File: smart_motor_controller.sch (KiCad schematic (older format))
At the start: 76 parts, among them J1 I2C_CONN_1, J10 USB_B_Micro, J11 M0_CONN, J12 M1_CONN, J13 M2_CONN, J14 M3_CONN, J2 I2C_CONN_2, J3 Conn_01x02, J4 Conn_02x05_Odd_Even, J5 Conn_01x02, J6 Conn_01x02, J7 Conn_01x02, J8 CAN_CONN, J9 Input 12V, Q1 AO3401A, SW1 SW_SPDT, U1 TPS5430DDA, U2 STM32F405RGT6, U3 USBLC6-2SC6, U4 DRV8871DDA, U5 DRV8871DDA, U6 DRV8871DDA, U7 DRV8871DDA

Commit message: V0.1.1 Removed fuse and AO3401A
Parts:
- removed F1: Polyfuse, Fuse:Fuse_1812_4532Metric, symbol Device:Polyfuse_Small
- removed Q1: AO3401A, Package_TO_SOT_SMD:SOT-23, symbol Transistor_FET:AO3401A
- R2, R3: footprint Resistor_SMD:R_0402_1005Metric -> Resistor_THT:R_Axial_DIN0204_L3.6mm_D1.6mm_P5.08mm_Horizontal; LCSC Part # C25879 -> (none)
- TP1: value 12V -> Vin
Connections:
- wire segments 172 -> 170
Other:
- moved on the sheet: C1, D1, D2, TP1
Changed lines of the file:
@@
 NoConn ~ 10800 1150
-$Comp
-L power:+12V #PWR0101
-U 1 1 602FED4E
-P 700 1000
-F 0 "#PWR0101" H 700 850 50  0001 C CNN
-F 1 "+12V" H 715 1173 50  0000 C CNN
-F 2 "" H 700 1000 50  0001 C CNN
-F 3 "" H 700 1000 50  0001 C CNN
-	1    700  1000
-	1    0    0    -1
-$EndComp
-$Comp
-L Device:Polyfuse_Small F1
-U 1 1 602FF711
-P 1500 1150
-F 0 "F1" V 1295 1150 50  0000 C CNN
-F 1 "Polyfuse" V 1386 1150 50  0000 C CNN
-F 2 "Fuse:Fuse_1812_4532Metric" H 1550 950 50  0001 L CNN
-F 3 "~" H 1500 1150 50  0001 C CNN
-F 4 "C495356" H 1500 1150 50  0001 C CNN "LCSC Part #"
-	1    1500 1150
-	0    1    1    0
-$EndComp
 $Comp
 L Connector:Screw_Terminal_01x02 J9
@@
 L power:+5V #PWR0110
 U 1 1 6038E68B
-P 2050 800
-F 0 "#PWR0110" H 2050 650 50  0001 C CNN
-F 1 "+5V" H 2065 973 50  0000 C CNN
-F 2 "" H 2050 800 50  0001 C CNN
-F 3 "" H 2050 800 50  0001 C CNN
-	1    2050 800
+P 1800 1050
+F 0 "#PWR0110" H 1800 900 50  0001 C CNN
+F 1 "+5V" H 1815 1223 50  0000 C CNN
+F 2 "" H 1800 1050 50  0001 C CNN
+F 3 "" H 1800 1050 50  0001 C CNN
+	1    1800 1050
 	1    0    0    -1
 $EndComp
@@
 F 0 "R2" H 4309 5646 50  0000 L CNN
 F 1 "2k2" H 4309 5555 50  0000 L CNN
-F 2 "Resistor_SMD:R_0402_1005Metric" H 4250 5600 50  0001 C CNN
+F 2 "Resistor_THT:R_Axial_DIN0204_L3.6mm_D1.6mm_P5.08mm_Horizontal" H 4250 5600 50  0001 C CNN
 F 3 "~" H 4250 5600 50  0001 C CNN
-F 4 "C25879" H 4250 5600 50  0001 C CNN "LCSC Part #"
+F 4 "" H 4250 5600 50  0001 C CNN "LCSC Part #"
 	1    4250 5600
 	1    0    0    -1
@@
 F 0 "R3" H 4609 5646 50  0000 L CNN
 F 1 "2k2" H 4609 5555 50  0000 L CNN
-F 2 "Resistor_SMD:R_0402_1005Metric" H 4550 5600 50  0001 C CNN
+F 2 "Resistor_THT:R_Axial_DIN0204_L3.6mm_D1.6mm_P5.08mm_Horizontal" H 4550 5600 50  0001 C CNN
 F 3 "~" H 4550 5600 50  0001 C CNN
-F 4 "C25879" H 4550 5600 50  0001 C CNN "LCSC Part #"
+F 4 "" H 4550 5600 50  0001 C CNN "LCSC Part #"
 	1    4550 5600
 	1    0    0    -1
@@
 L Device:C_Small C1
 U 1 1 60354332
-P 2250 1350
-F 0 "C1" H 2342 1396 50  0000 L CNN
-F 1 "10u" H 2342 1305 50  0000 L CNN
-F 2 "Capacitor_SMD:C_1206_3216Metric" H 2250 1350 50  0001 C CNN
-F 3 "~" H 2250 1350 50  0001 C CNN
-F 4 "C13585" H 2250 1350 50  0001 C CNN "LCSC Part #"
-	1    2250 1350
+P 2000 1600
+F 0 "C1" H 2092 1646 50  0000 L CNN
+F 1 "10u" H 2092 1555 50  0000 L CNN
+F 2 "Capacitor_SMD:C_1206_3216Metric" H 2000 1600 50  0001 C CNN
+F 3 "~" H 2000 1600 50  0001 C CNN
+F 4 "C13585" H 2000 1600 50  0001 C CNN "LCSC Part #"
+	1    2000 1600
 	1    0    0    -1
 $EndComp
@@
 Text GLabel 4200 1000 0    50   Input ~ 0
 BACK_IN
-Text GLabel 2400 1150 2    50   Input ~ 0
+Text GLabel 2150 1400 2    50   Input ~ 0
 BACK_IN
 $Comp
 L power:GND #PWR0117
 U 1 1 6037A407
-P 2250 1450
-F 0 "#PWR0117" H 2250 1200 50  0001 C CNN
-F 1 "GND" H 2255 1277 50  0000 C CNN
-F 2 "" H 2250 1450 50  0001 C CNN
-F 3 "" H 2250 1450 50  0001 C CNN
-	1    2250 1450
-	1    0    0    -1
-$EndComp
-Wire Wire Line
-	2400 1150 2250 1150
-Wire Wire Line
-	2250 1150 2250 1250
+P 2000 1700
+F 0 "#PWR0117" H 2000 1450 50  0001 C CNN
+F 1 "GND" H 2005 1527 50  0000 C CNN
+F 2 "" H 2000 1700 50  0001 C CNN
+F 3 "" H 2000 1700 50  0001 C CNN
+	1    2000 1700
+	1    0    0    -1
+$EndComp
+Wire Wire Line
+	2150 1400 2000 1400
+Wire Wire Line
+	2000 1400 2000 1500
 Text GLabel 3300 850  0    50   Input ~ 0
 BACK_IN
@@
 Wire Wire Line
 	3800 3800 3950 3800
-Wire Wire Line
-	700  1000 700  1150
-Connection ~ 2250 1150
+Connection ~ 2000 1400
 $Comp
 L Device:D_Schottky_Small D1
 U 1 1 603C17FB
-P 2050 1000
-F 0 "D1" V 2250 850 50  0000 L CNN
-F 1 "B5819W" V 2150 650 50  0000 L CNN
-F 2 "Diode_SMD:D_SOD-123" V 2050 1000 50  0001 C CNN
-F 3 "~" V 2050 1000 50  0001 C CNN
-F 4 "C8598" H 2050 1000 50  0001 C CNN "LCSC Part #"
-	1    2050 1000
+P 1800 1250
+F 0 "D1" V 2000 1100 50  0000 L CNN
+F 1 "B5819W" V 1900 900 50  0000 L CNN
+F 2 "Diode_SMD:D_SOD-123" V 1800 1250 50  0001 C CNN
+F 3 "~" V 1800 1250 50  0001 C CNN
+F 4 "C8598" H 1800 1250 50  0001 C CNN "LCSC Part #"
+	1    1800 1250
 	0    -1   -1   0
 $EndComp
 Wire Wire Line
-	2050 1100 2050 1150
-Wire Wire Line
-	2050 1150 2250 1150
-Wire Wire Line
-	2050 800  2050 900
+	1800 1350 1800 1400
+Wire Wire Line
+	1800 1400 2000 1400
+Wire Wire Line
+	1800 1050 1800 1150
 Text GLabel 10200 4150 2    50   Input ~ 0
 VM
@@
 	6500 4500 6500 4600
 Connection ~ 6500 4600
-Wire Wire Line
-	700  1150 850  1150
-$Comp
-L Device:D_Schottky_Small D2
-U 1 1 603C3D54
-P 1900 1150
-F 0 "D2" H 1950 1050 50  0000 L CNN
-F 1 "B5819W" H 1750 1250 50  0000 L CNN
-F 2 "Diode_SMD:D_SOD-123" V 1900 1150 50  0001 C CNN
-F 3 "~" V 1900 1150 50  0001 C CNN
-F 4 "C8598" H 1900 1150 50  0001 C CNN "LCSC Part #"
-	1    1900 1150
-	-1   0    0    1
-$EndComp
-Text GLabel 1750 1450 2    50   Input ~ 0
-VM
-Wire Wire Line
-	1600 1150 1700 1150
-Connection ~ 1700 1150
-Wire Wire Line
-	1700 1150 1800 1150
-Wire Wire Line
-	2000 1150 2050 1150
-Connection ~ 2050 1150
-Wire Wire Line
-	1700 1450 1750 1450
-Wire Wire Line
-	1700 1150 1700 1450
 Text GLabel 2900 6500 2    50   Input ~ 0
 GPIO0
@@
 	10150 5450 10150 5500
 $Comp
-L power:GND #PWR0133
-U 1 1 60394456
-P 1050 1450
-F 0 "#PWR0133" H 1050 1200 50  0001 C CNN
-F 1 "GND" H 1055 1277 50  0000 C CNN
-F 2 "" H 1050 1450 50  0001 C CNN
-F 3 "" H 1050 1450 50  0001 C CNN
-	1    1050 1450
-	1    0    0    -1
-$EndComp
-$Comp
-L Transistor_FET:AO3401A Q1
-U 1 1 6039186B
-P 1050 1250
-F 0 "Q1" V 1392 1250 50  0000 C CNN
-F 1 "AO3401A" V 1301 1250 50  0000 C CNN
-F 2 "Package_TO_SOT_SMD:SOT-23" H 1250 1175 50  0001 L CIN
-F 3 "http://www.aosmd.com/pdfs/datasheet/AO3401A.pdf" H 1050 1250 50  0001 L CNN
-F 4 "C693260" H 1050 1250 50  0001 C CNN "LCSC Part #"
-	1    1050 1250
-	0    -1   -1   0
-$EndComp
-Connection ~ 1350 1150
-Wire Wire Line
-	1350 1150 1400 1150
-Wire Wire Line
-	1250 1150 1350 1150
-Wire Wire Line
-	1350 1150 1350 1300
-$Comp
-L Connector:TestPoint_Small TP1
-U 1 1 604A4E02
-P 1350 1300
-F 0 "TP1" H 1398 1346 50  0000 L CNN
-F 1 "12V" H 1398 1255 50  0000 L CNN
-F 2 "TestPoint:TestPoint_Pad_D2.0mm" H 1550 1300 50  0001 C CNN
-F 3 "~" H 1550 1300 50  0001 C CNN
-	1    1350 1300
-	1    0    0    -1
-$EndComp
-$Comp
 L Connector:TestPoint_Small TP2
 U 1 1 606A33A8
@@
 Text GLabel 5200 1200 2    50   Input ~ 0
 BACK_PH
+$Comp
+L power:+12V #PWR0101
+U 1 1 602FED4E
+P 800 1050
+F 0 "#PWR0101" H 800 900 50  0001 C CNN
+F 1 "+12V" H 815 1223 50  0000 C CNN
+F 2 "" H 800 1050 50  0001 C CNN
+F 3 "" H 800 1050 50  0001 C CNN
+	1    800  1050
+	1    0    0    -1
+$EndComp
+Text GLabel 1100 1700 2    50   Input ~ 0
+VM
+Wire Wire Line
+	1050 1700 1100 1700
+$Comp
+L Device:D_Schottky_Small D2
+U 1 1 603C3D54
+P 1250 1400
+F 0 "D2" H 1300 1300 50  0000 L CNN
+F 1 "B5819W" H 1100 1500 50  0000 L CNN
+F 2 "Diode_SMD:D_SOD-123" V 1250 1400 50  0001 C CNN
+F 3 "~" V 1250 1400 50  0001 C CNN
+F 4 "C8598" H 1250 1400 50  0001 C CNN "LCSC Part #"
+	1    1250 1400
+	-1   0    0    1
+$EndComp
+Wire Wire Line
+	1050 1400 1150 1400
+Connection ~ 1050 1400
+Wire Wire Line
+	1050 1400 1050 1700
+$Comp
+L Connector:TestPoint_Small TP1
+U 1 1 604A4E02
+P 1600 1600
+F 0 "TP1" H 1648 1646 50  0000 L CNN
+F 1 "Vin" H 1648 1555 50  0000 L CNN
+F 2 "TestPoint:TestPoint_Pad_D2.0mm" H 1800 1600 50  0001 C CNN
+F 3 "~" H 1800 1600 50  0001 C CNN
+	1    1600 1600
+	1    0    0    -1
+$EndComp
+Wire Wire Line
+	800  1050 800  1400
+Wire Wire Line
+	1350 1400 1600 1400
+Connection ~ 1800 1400
+Wire Wire Line
+	1600 1600 1600 1400
+Connection ~ 1600 1400
+Wire Wire Line
+	1600 1400 1800 1400
+Wire Wire Line
+	800  1400 1050 1400
 $EndSCHEMATC

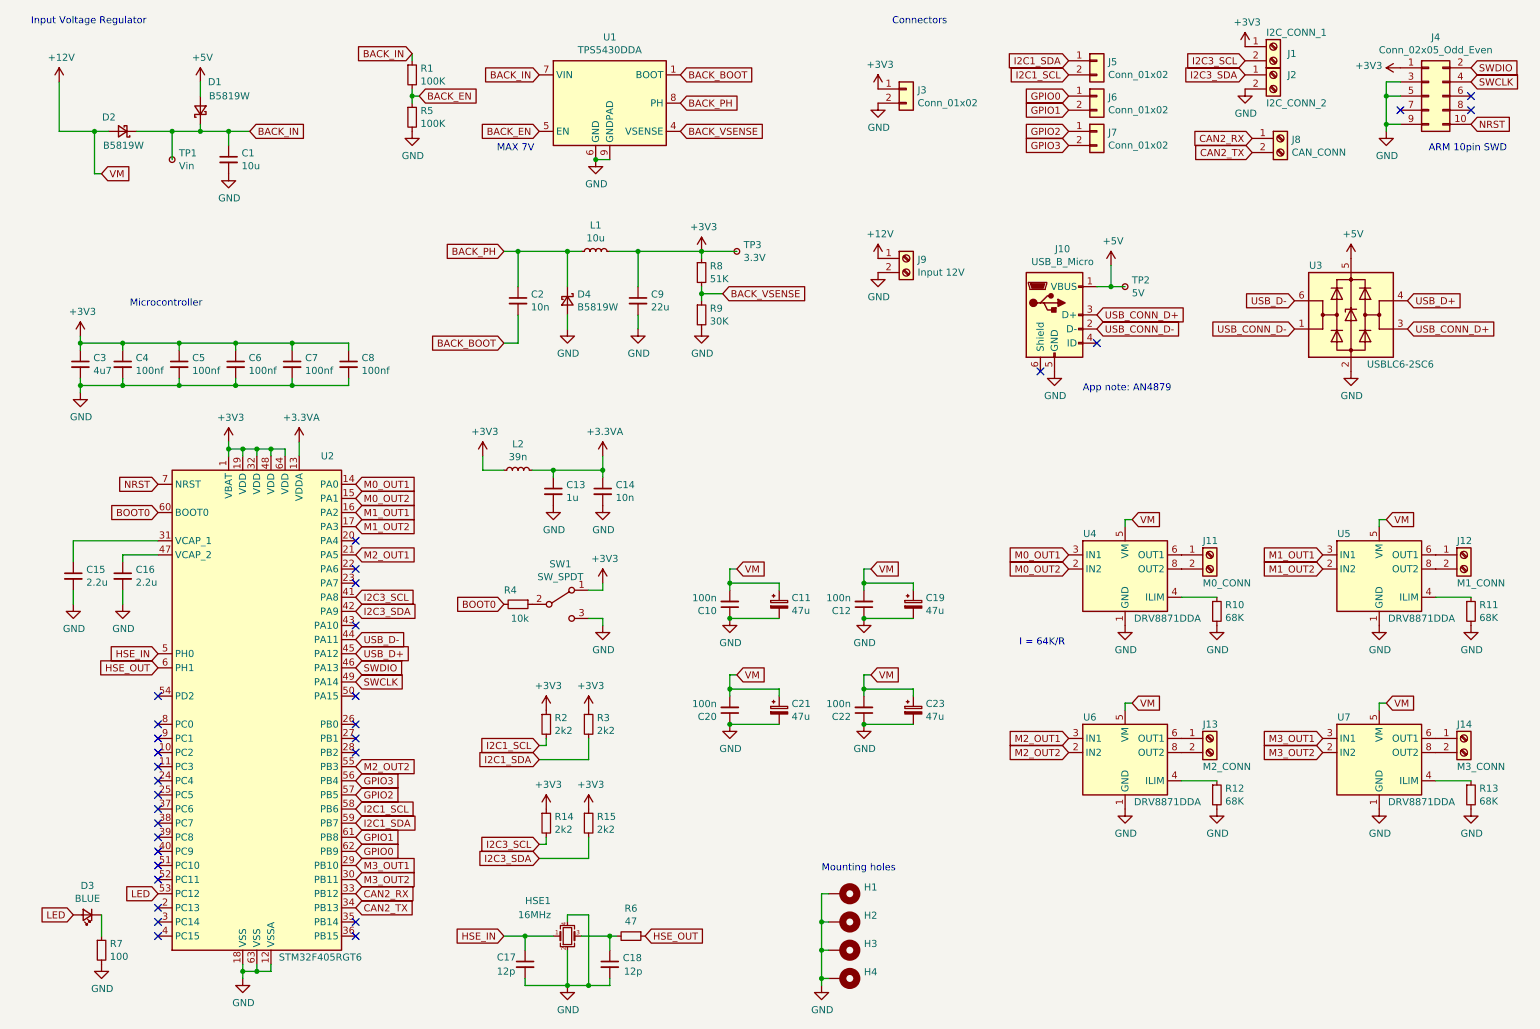
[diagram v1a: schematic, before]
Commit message: First draft
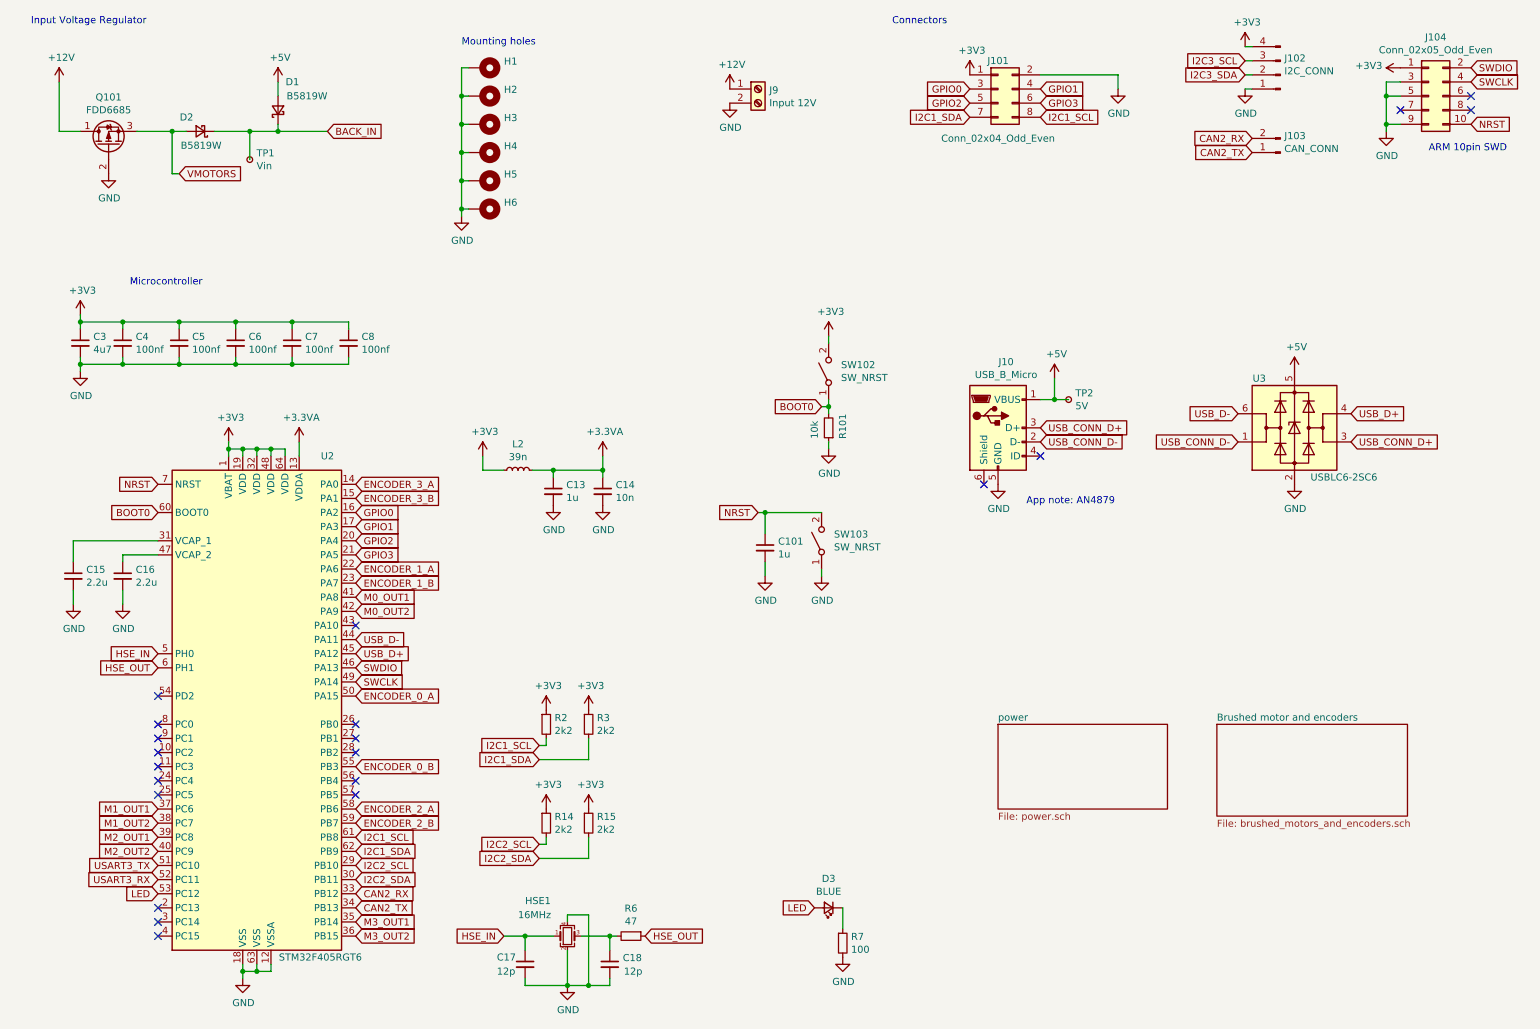
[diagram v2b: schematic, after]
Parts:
- removed C1: 10u, Capacitor_SMD:C_1206_3216Metric, symbol Device:C_Small
- removed C10, C12, C20, C22: 100n, Capacitor_SMD:C_0603_1608Metric, symbol Device:C_Small
- removed C11, C19, C21, C23: 47u, Capacitor_THT:CP_Radial_D5.0mm_P2.00mm, symbol Device:CP_Small
- removed C2: 10n, Capacitor_SMD:C_0402_1005Metric, symbol Device:C_Small
- removed C9: 22u, Capacitor_SMD:C_0603_1608Metric, symbol Device:C_Small
- removed D4: B5819W, Diode_SMD:D_SOD-123, symbol Device:D_Schottky_Small
- removed J1: I2C_CONN_1, VsReality_Footprints:DB128L_5.08_2P_GN_S, symbol Connector:Screw_Terminal_01x02
- removed J11: M0_CONN, VsReality_Footprints:DB128L_5.08_2P_GN_S, symbol Connector:Screw_Terminal_01x02
- removed J12: M1_CONN, VsReality_Footprints:DB128L_5.08_2P_GN_S, symbol Connector:Screw_Terminal_01x02
- removed J13: M2_CONN, VsReality_Footprints:DB128L_5.08_2P_GN_S, symbol Connector:Screw_Terminal_01x02
- removed J14: M3_CONN, VsReality_Footprints:DB128L_5.08_2P_GN_S, symbol Connector:Screw_Terminal_01x02
- removed J2: I2C_CONN_2, VsReality_Footprints:DB128L_5.08_2P_GN_S, symbol Connector:Screw_Terminal_01x02
- removed J3, J5, J6, J7: Conn_01x02, Connector_PinHeader_2.54mm:PinHeader_1x02_P2.54mm_Vertical, symbol Connector_Generic:Conn_01x02
- removed J8: CAN_CONN, VsReality_Footprints:DB128L_5.08_2P_GN_S, symbol Connector:Screw_Terminal_01x02
- removed L1: 10u, Inductor_SMD:L_Sunlord_MWSA0518_5.4x5.2mm, symbol Device:L_Small
- removed R1, R5: 100K, Resistor_SMD:R_0402_1005Metric, symbol Device:R_Small
- removed R10, R11, R12, R13: 68K, Resistor_SMD:R_0402_1005Metric, symbol Device:R_Small
- removed R4: 10k, Resistor_SMD:R_0402_1005Metric, symbol Device:R_Small
- removed R8: 51K, Resistor_SMD:R_0603_1608Metric, symbol Device:R_Small
- removed R9: 30K, Resistor_SMD:R_0603_1608Metric, symbol Device:R_Small
- removed SW1: SW_SPDT, VsReality_Footprints:SW_SPDT, symbol Switch:SW_SPDT
- removed TP3: 3.3V, TestPoint:TestPoint_Pad_D1.5mm, symbol Connector:TestPoint_Small
- removed U1: TPS5430DDA, Package_SO:TI_SO-PowerPAD-8_ThermalVias, symbol Regulator_Switching:TPS5430DDA
- removed U4, U5, U6, U7: DRV8871DDA, Package_SO:Texas_HTSOP-8-1EP_3.9x4.9mm_P1.27mm_EP2.95x4.9mm_Mask2.4x3.1mm_ThermalVias, symbol Driver_Motor:DRV8871DDA
- added C101: 1u, Capacitor_SMD:C_0402_1005Metric, symbol Device:C_Small
- added H5, H6: MountingHole_Pad, MountingHole:MountingHole_2.7mm_M2.5_Pad, symbol Mechanical:MountingHole_Pad
- added J101: Conn_02x04_Odd_Even, Connector_PinHeader_2.54mm:PinHeader_2x04_P2.54mm_Vertical, symbol Connector_Generic:Conn_02x04_Odd_Even
- added J102: I2C_CONN, Connector_JST:JST_PH_S4B-PH-SM4-TB_1x04-1MP_P2.00mm_Horizontal, symbol Connector:Conn_01x04_Male
- added J103: CAN_CONN, Connector_JST:JST_PH_S2B-PH-SM4-TB_1x02-1MP_P2.00mm_Horizontal, symbol Connector:Conn_01x02_Male
- added Q101: FDD6685, Package_TO_SOT_SMD:TO-252-2, symbol VsReality_Symbols:FDD6685
- added R101: 10k, Resistor_SMD:R_0402_1005Metric, symbol Device:R_Small
- added SW102, SW103: SW_NRST, symbol Switch:SW_SPST
- H1, H2, H3, H4: footprint MountingHole:MountingHole_4.3mm_M4_Pad_Via -> MountingHole:MountingHole_2.7mm_M2.5_Pad
- renumbered J4 to J104
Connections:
- net +12V: now also Q101.1 (D); no longer D2.2 (A)
- net +3V3: now also J101.1 (Pin_1), J102.4 (Pin_4), SW102.2 (B)
- net BOOT0: now also R101.2, SW102.1 (A)
- net CAN2_RX: now also J103.2 (Pin_2)
- net CAN2_TX: now also J103.1 (Pin_1)
- net GND: now also C101.2, H5.1, H6.1, J101.2 (Pin_2), J102.1 (Pin_1), Q101.2 (G), R101.1, SW103.1 (A)
- net GPIO0: now also U2.16 (PA2), J101.3 (Pin_3); no longer U2.62 (PB9)
- net GPIO1: now also U2.17 (PA3), J101.4 (Pin_4); no longer U2.61 (PB8)
- net GPIO2: now also U2.20 (PA4), J101.5 (Pin_5); no longer U2.57 (PB5)
- net GPIO3: now also U2.21 (PA5), J101.6 (Pin_6); no longer U2.56 (PB4)
- net I2C1_SCL: now also U2.61 (PB8), J101.8 (Pin_8); no longer U2.58 (PB6)
- net I2C1_SDA: now also U2.62 (PB9), J101.7 (Pin_7); no longer U2.59 (PB7)
- net I2C3_SCL: now also J102.3 (Pin_3); no longer R14.2, U2.41 (PA8)
- net I2C3_SDA: now also J102.2 (Pin_2); no longer R15.2, U2.42 (PA9)
- net M0_OUT1: now also U2.41 (PA8); no longer U2.14 (PA0)
- net M0_OUT2: now also U2.42 (PA9); no longer U2.15 (PA1)
- net M1_OUT1: now also U2.37 (PC6); no longer U2.16 (PA2)
- net M1_OUT2: now also U2.38 (PC7); no longer U2.17 (PA3)
- net M2_OUT1: now also U2.39 (PC8); no longer U2.21 (PA5)
- net M2_OUT2: now also U2.40 (PC9); no longer U2.55 (PB3)
- net M3_OUT1: now also U2.35 (PB14); no longer U2.29 (PB10)
- net M3_OUT2: now also U2.36 (PB15); no longer U2.30 (PB11)
- net NRST: now also C101.1, SW103.2 (B)
- net ENCODER_1_A: now reaches U2.22 (PA6)
- net ENCODER_1_B: now reaches U2.23 (PA7)
- net ENCODER_0_A: now reaches U2.50 (PA15)
- net USART3_TX: now reaches U2.51 (PC10)
- net USART3_RX: now reaches U2.52 (PC11)
- new net ENCODER_0_B: U2.55 (PB3)
- new net ENCODER_2_A: U2.58 (PB6)
- new net ENCODER_2_B: U2.59 (PB7)
- new net ENCODER_3_A: U2.14 (PA0)
- new net ENCODER_3_B: U2.15 (PA1)
- new net I2C2_SCL: R14.2, U2.29 (PB10)
- new net I2C2_SDA: R15.2, U2.30 (PB11)
- new net VMOTORS: D2.2 (A), Q101.3 (S)
- no-connect marks 31 -> 21
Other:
- note removed: "I = 64K/R"
- note removed: "MAX 7V"
- moved on the sheet: C3, C4, C5, C6, C7, C8, D1, D2, D3, H1, H2, H3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
